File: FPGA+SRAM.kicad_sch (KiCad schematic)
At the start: 0 parts

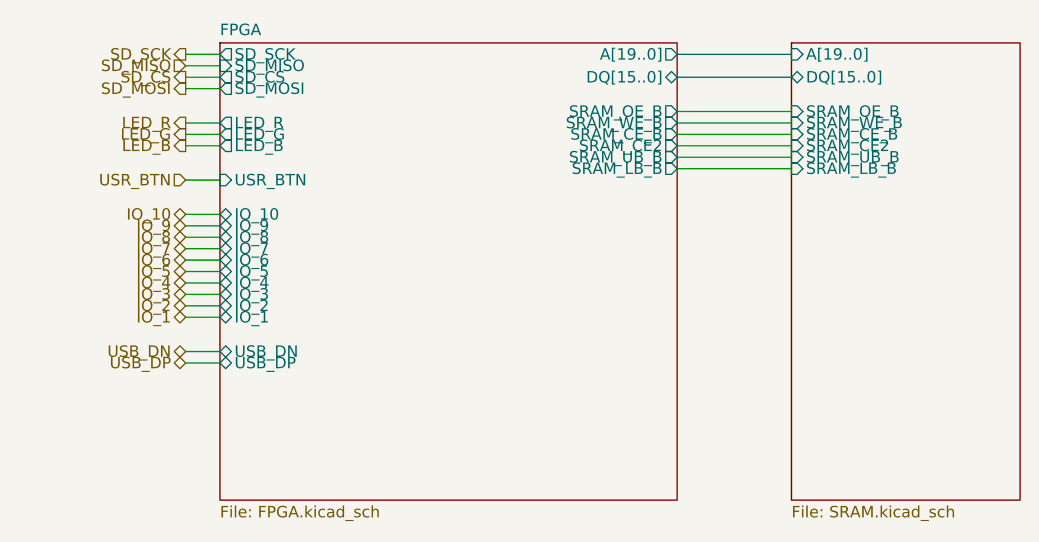
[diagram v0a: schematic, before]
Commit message: Power routed. Saving before reworking ICE40 pins to optimize layout
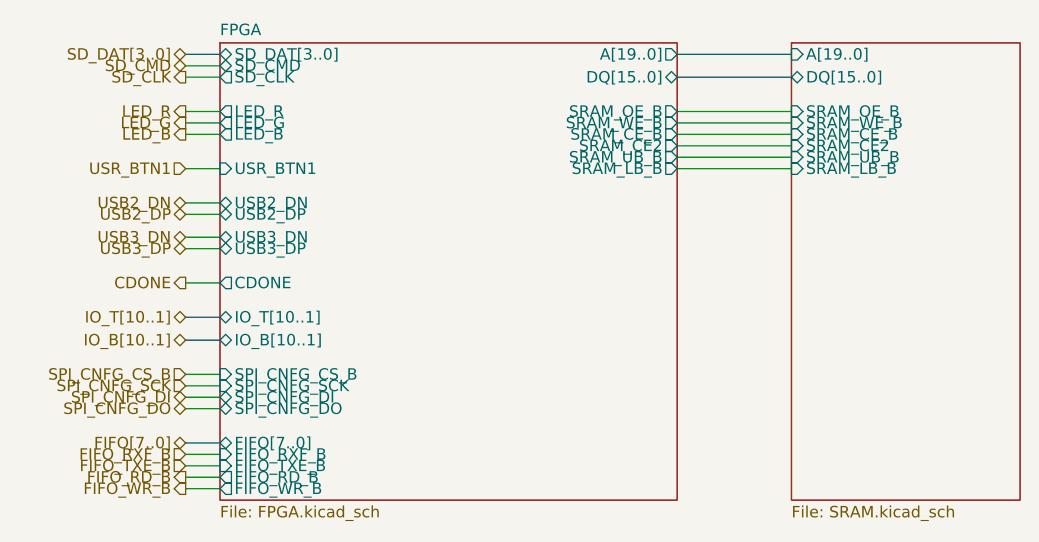
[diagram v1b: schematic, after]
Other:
- sheet FPGA ports: added CDONE, FIFO[7..0], FIFO_RD_B, FIFO_RXF_B, FIFO_TXE_B, FIFO_WR_B, IO_B[10..1], IO_T[10..1], SD_CLK, SD_CMD, SD_DAT[3..0], SPI_CNFG_CS_B, SPI_CNFG_DI, SPI_CNFG_DO, SPI_CNFG_SCK, USB2_DN, USB2_DP, USB3_DN, USB3_DP, USR_BTN1; removed IO_1, IO_10, IO_2, IO_3, IO_4, IO_5, IO_6, IO_7, IO_8, IO_9, SD_CS, SD_MISO, SD_MOSI, SD_SCK, USB_DN, USB_DP, USR_BTN
